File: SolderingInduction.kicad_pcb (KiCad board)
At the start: 4 copper layers, 68.9 x 37.6 mm, 57 parts, among them J1 MC-307, J3 RBP_GPIO_CONN, SW1 SW_Push, SW2 SW_Push, SW3 SW_Push, SW4 SW_Push, SW5 SW_Push, SW6 SW_Push, SW7 SW_Push, SW8 SW_Push, U1 SPX2920M3-3.3_SOT223, U3 W25Q32JVZP, U4 RP2040, Y1 X322512MMB4SI

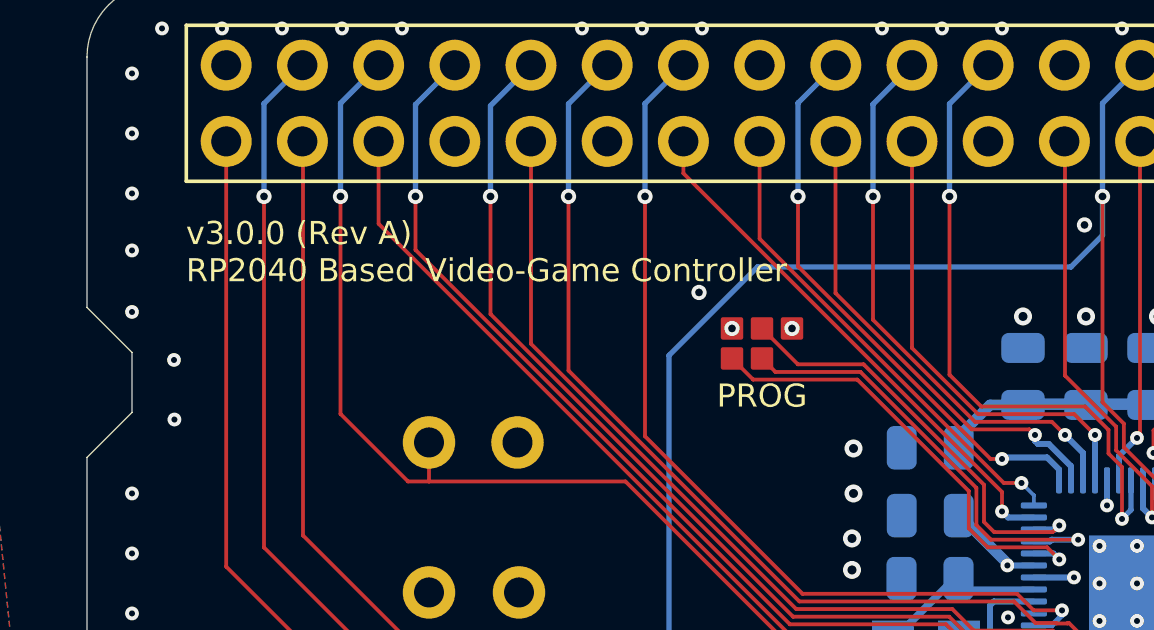
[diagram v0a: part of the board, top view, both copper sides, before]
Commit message: Frog
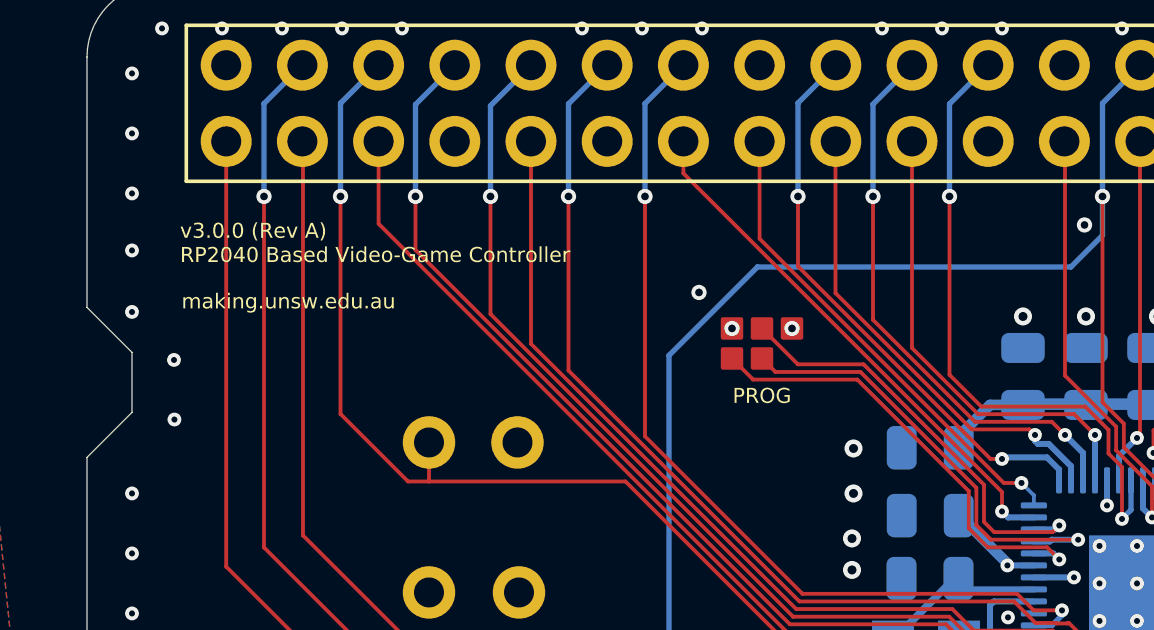
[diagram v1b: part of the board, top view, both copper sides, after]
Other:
- board text added: "making.unsw.edu.au"
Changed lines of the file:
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@@
   (gr_line (start 92.45 92.45) (end 156.467588 92.517588) (layer "Edge.Cuts") (width 0.01))
   (gr_line (start 158.917588 90.067588) (end 158.942588 57.417588) (layer "Edge.Cuts") (width 0.01))
-  (gr_text "v3.0.0 (Rev A)\nRP2040 Based Video-Game Controller" (at 93.3 63.95) (layer "F.SilkS")
-    (effects (font (size 0.77 0.77) (thickness 0.1925)) (justify left))
+  (gr_text "v3.0.0 (Rev A)\nRP2040 Based Video-Game Controller" (at 93.1 63.65) (layer "F.SilkS")
+    (effects (font (size 0.5 0.5) (thickness 0.125)) (justify left))
+  )
+  (gr_text "making.unsw.edu.au" (at 93.15 65.6) (layer "F.SilkS")
+    (effects (font (size 0.5 0.5) (thickness 0.125)) (justify left))
   )
   (gr_text "PROG" (at 112.5 68.75) (layer "F.SilkS")
-    (effects (font (size 0.77 0.77) (thickness 0.15)))
+    (effects (font (size 0.5 0.5) (thickness 0.125)))
   )
   (gr_text "Todo:\n* Tune DRC \n	- Ensure the scripted DRC cons don't conflict \n	- soldermask expansion \n	- silkscreen reqs \n	- trace clearances \n* Tune and run ERC\n* Clean up trace width / clearances\n* Clean up board dimensions \n* Confirm testpoints to 1mm spacing grid\n* Adjust all via sizes \n* Update schematic to 1117-3v3 \n* Redo power layout \n* Cleanup 3v3 and 1v2 power traces \n* Clean up zones \n* Clean up schematic \n* Route GPIO \n* Double check LED \n* Check if buttons can be diagonalized \n* Clean up D-pad layout\n* Clean up SWD footprint \n* check optimality of via placements \n* Draw out grid for vias \n* run traces to fan-in fan-out \n* Check clearances and trace widths \n* Check ground flow paths \n* Check button footprints \n* Check river routing consistency \n* Check USB interface layout \n* Clean up silkscreen \n* Change QR code\n* Clean up oscillator \n* Clean up passives \n* Ensure all decoupling caps grounded properly \n* Map GPIO \n* Connect up GPIO \n* Check accessibility \n* Comply with JLC SMT reqs" (at 166.8 69.9352) (layer "Cmts.User")
